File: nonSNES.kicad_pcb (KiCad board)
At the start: 4 copper layers, 185.4 x 160 mm, 19 parts, among them J1 Jack-DC, P1 CASSETTE, P3 Conn_01x02_Male, T1 L_Coupled, U1 CPU, U12 L7805, U2 PQFP-100_14x20mm_P0.65mm, U3 PQFP-100_14x20mm_P0.65mm, U4 MS62256CL-10FC, U5 MS62256CL-10FC

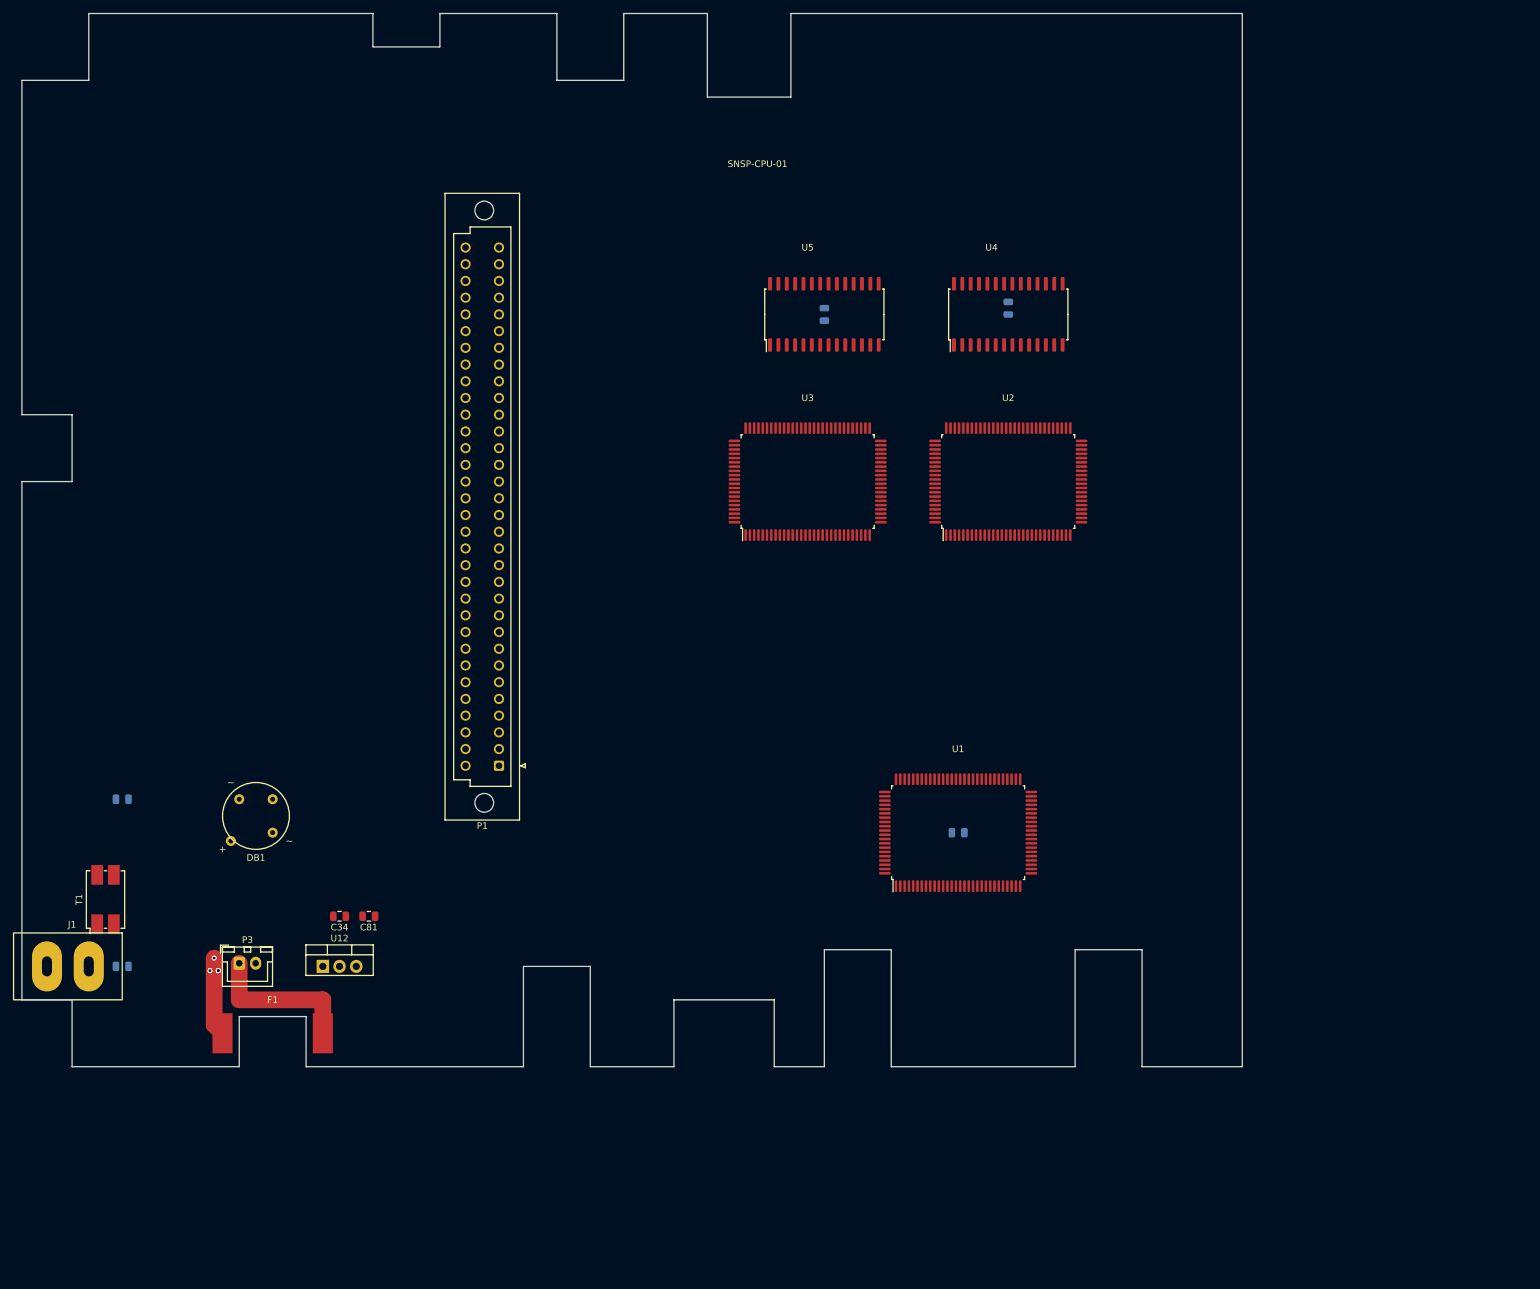
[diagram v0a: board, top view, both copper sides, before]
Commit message: get board outline right
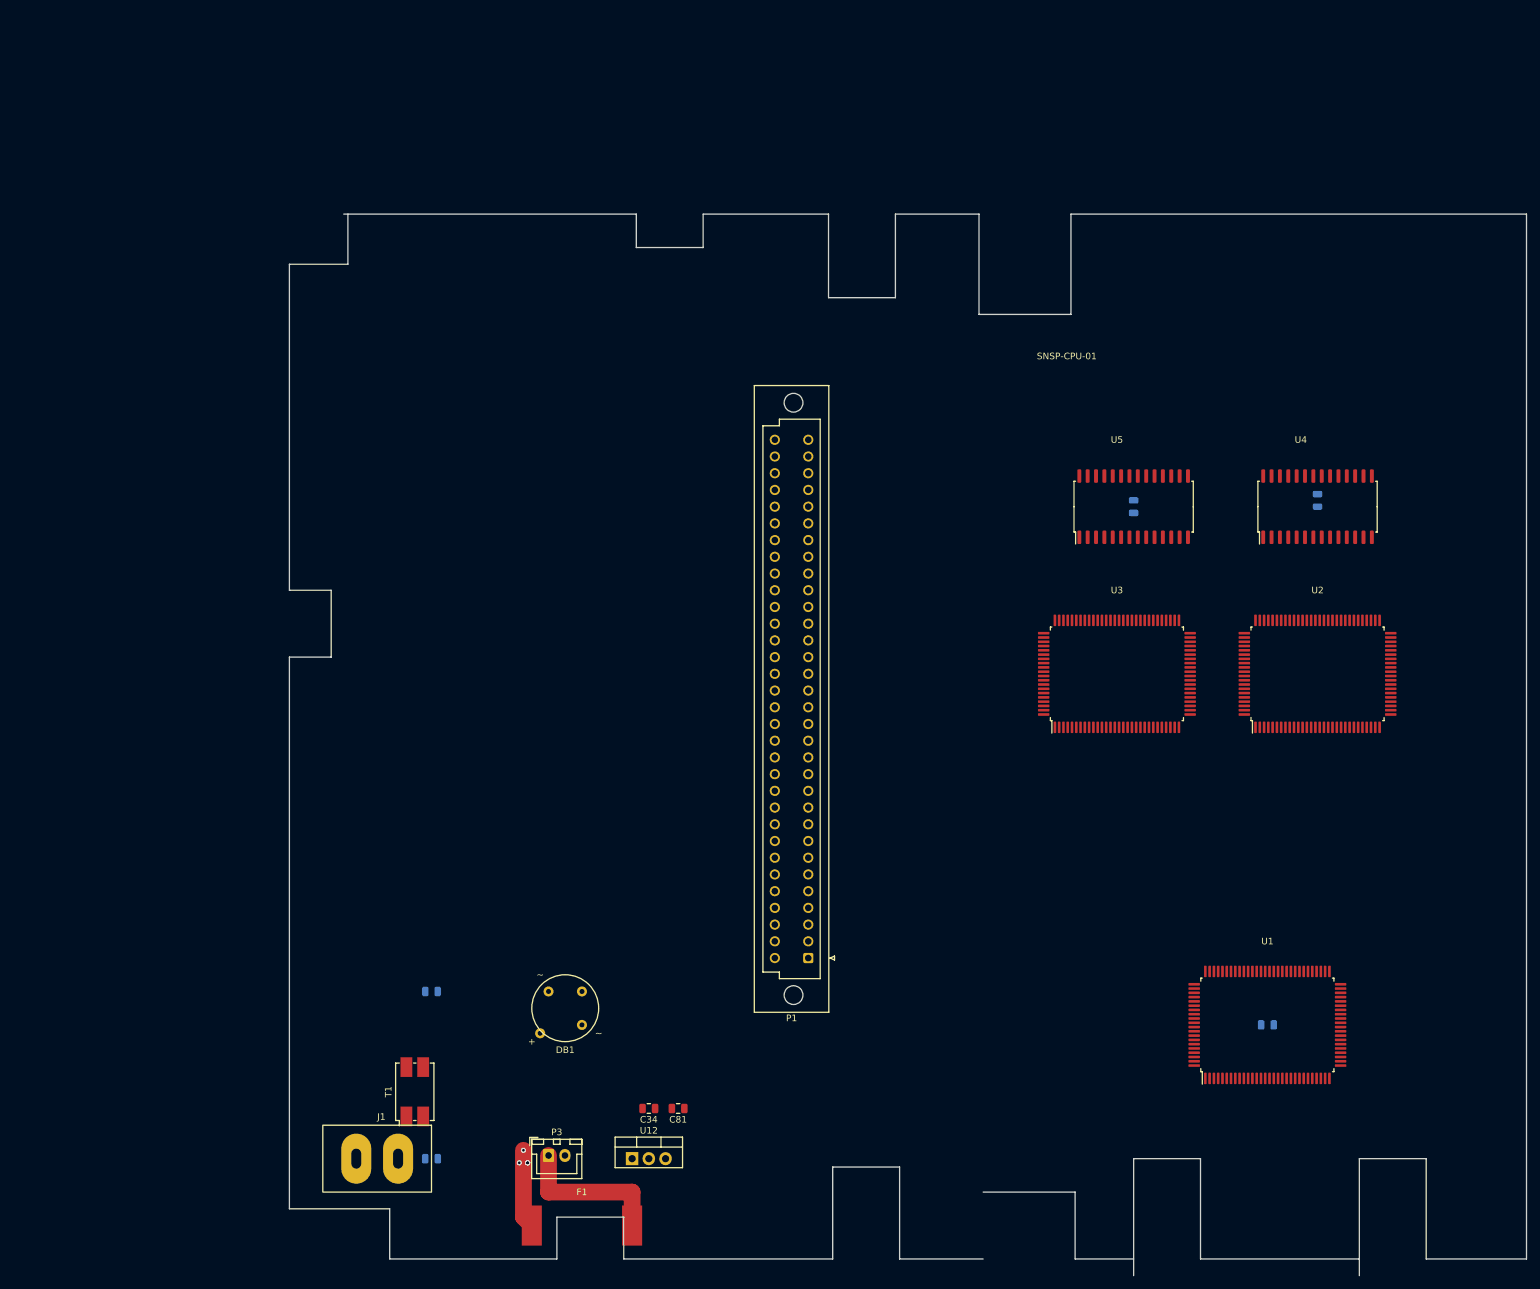
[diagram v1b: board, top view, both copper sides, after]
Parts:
- moved C93 55.3 mm to (212.1, 176.5)
- moved C95 55.3 mm to (191.8, 97.8)
- moved C97 55.3 mm to (219.7, 96.8)
- moved P1 55.3 mm to (142.3, 166.4)
- moved U1 55.3 mm to (212.1, 176.5)
- moved U4 55.3 mm to (219.7, 97.8)
- moved U5 55.3 mm to (191.8, 97.8)
- moved C30 55.3 mm to (85.1, 196.8)
- moved P3 55.3 mm to (102.9, 196.4)
- moved U2 55.3 mm to (219.7, 123.2)
- moved C81 55.3 mm to (122.6, 189.2)
- moved DB1 55.3 mm to (105.4, 174.0)
- moved J1 55.3 mm to (77.5, 196.8)
- moved T1 55.3 mm to (82.5, 186.7)
- moved U12 55.3 mm to (115.6, 196.8)
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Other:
- board size 185.4 x 160 mm -> 188 x 161.3 mm
